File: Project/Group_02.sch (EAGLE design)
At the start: 29 parts, among them J1 POWER_JACKPTH_LOCK, U1 +12v

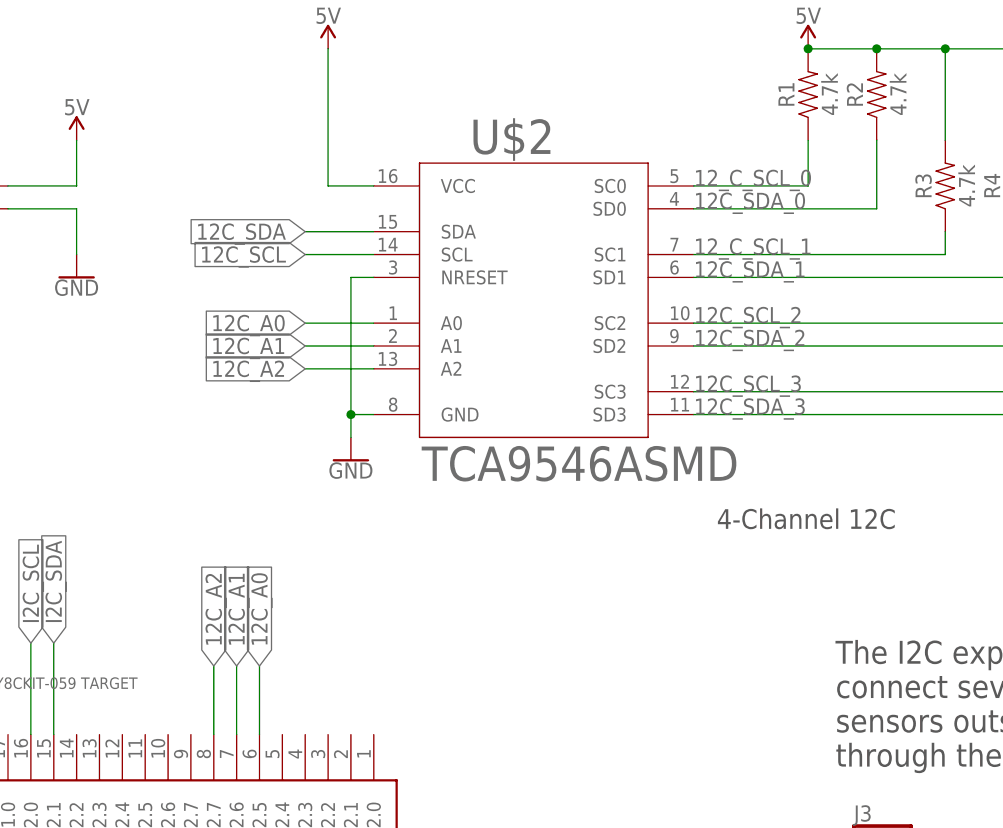
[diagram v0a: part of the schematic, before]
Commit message: PCB completa
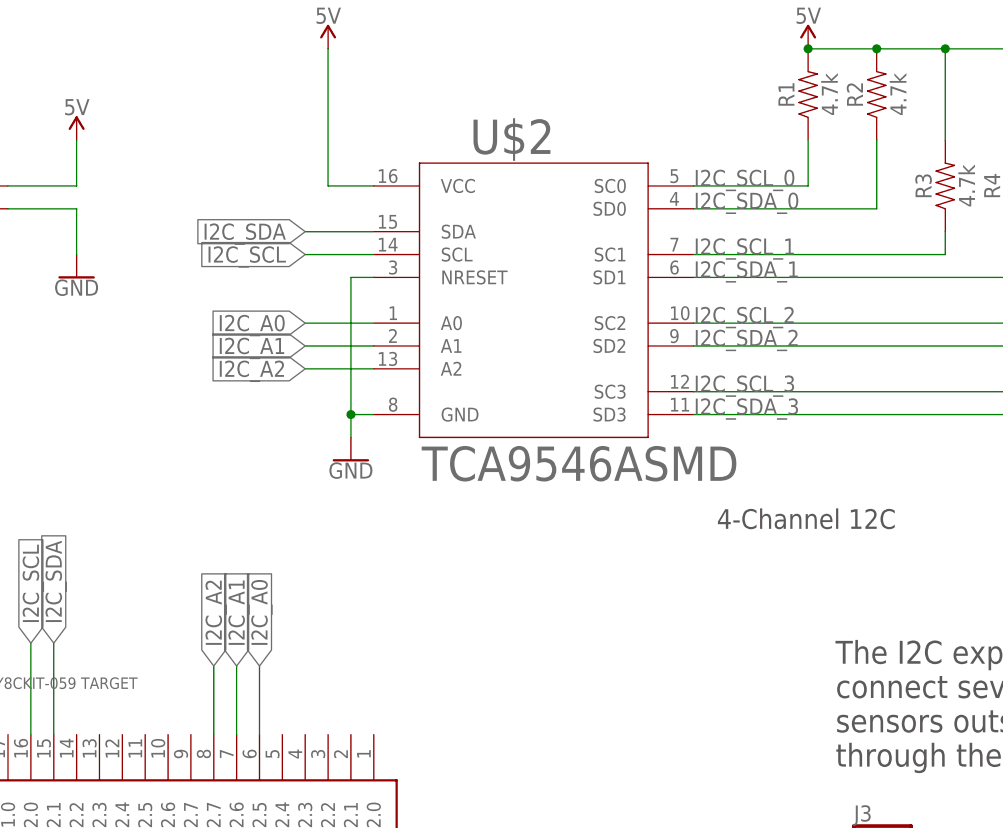
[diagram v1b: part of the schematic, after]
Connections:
- net 12C_A0 renamed I2C_A0
- net 12C_A1 renamed I2C_A1
- net 12C_A2 renamed I2C_A2
- removed net 12C_SCL: U$2.SCL
- removed net 12C_SCL_2: R5.1, U$2.SC2
- removed net 12C_SCL_3: R7.1, U$2.SC3
- removed net 12C_SDA: U$2.SDA
- removed net 12C_SDA_0: R2.1, U$2.SD0
- removed net 12C_SDA_1: R4.1, U$2.SD1
- removed net 12C_SDA_2: R6.1, U$2.SD2
- removed net 12C_SDA_3: R8.1, U$2.SD3
- removed net 12_C_SCL_0: R1.1, U$2.SC0
- removed net 12_C_SCL_1: R3.1, U$2.SC1
- net I2C_SCL: now also U$2.SCL
- net I2C_SCL_0: now also R1.1, U$2.SC0
- net I2C_SCL_1: now also R3.1, U$2.SC1
- net I2C_SCL_2: now also R5.1, U$2.SC2
- net I2C_SCL_3: now also R7.1, U$2.SC3
- net I2C_SDA: now also U$2.SDA
- net I2C_SDA_0: now also R2.1, U$2.SD0
- net I2C_SDA_1: now also R4.1, U$2.SD1
- net I2C_SDA_2: now also R6.1, U$2.SD2
- net I2C_SDA_3: now also R8.1, U$2.SD3
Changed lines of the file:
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@@
 <label x="243.84" y="40.64" size="1.778" layer="95" xref="yes"/>
+</segment>
+<segment>
+<pinref part="U$2" gate="G$1" pin="SD3"/>
+<pinref part="R8" gate="G$1" pin="1"/>
+<wire x1="205.74" y1="137.16" x2="271.78" y2="137.16" width="0.1524" layer="91"/>
+<wire x1="271.78" y1="137.16" x2="271.78" y2="142.24" width="0.1524" layer="91"/>
+<label x="205.74" y="137.16" size="1.778" layer="95"/>
 </segment>
 </net>
@@
 <label x="243.84" y="43.18" size="1.778" layer="95" xref="yes"/>
 </segment>
+<segment>
+<pinref part="U$2" gate="G$1" pin="SC3"/>
+<pinref part="R7" gate="G$1" pin="1"/>
+<wire x1="205.74" y1="139.7" x2="264.16" y2="139.7" width="0.1524" layer="91"/>
+<wire x1="264.16" y1="139.7" x2="264.16" y2="142.24" width="0.1524" layer="91"/>
+<label x="205.74" y="139.7" size="1.778" layer="95"/>
+</segment>
 </net>
 <net name="I2C_SDA_2" class="0">
@@
 <label x="243.84" y="55.88" size="1.778" layer="95" xref="yes"/>
 </segment>
+<segment>
+<pinref part="U$2" gate="G$1" pin="SD2"/>
+<pinref part="R6" gate="G$1" pin="1"/>
+<wire x1="205.74" y1="144.78" x2="256.54" y2="144.78" width="0.1524" layer="91"/>
+<wire x1="256.54" y1="144.78" x2="256.54" y2="149.86" width="0.1524" layer="91"/>
+<label x="205.74" y="144.78" size="1.778" layer="95"/>
+</segment>
 </net>
 <net name="I2C_SCL_2" class="0">
@@
 <label x="243.84" y="58.42" size="1.778" layer="95" xref="yes"/>
 </segment>
+<segment>
+<pinref part="U$2" gate="G$1" pin="SC2"/>
+<pinref part="R5" gate="G$1" pin="1"/>
+<wire x1="205.74" y1="147.32" x2="248.92" y2="147.32" width="0.1524" layer="91"/>
+<wire x1="248.92" y1="147.32" x2="248.92" y2="149.86" width="0.1524" layer="91"/>
+<label x="205.74" y="147.32" size="1.778" layer="95"/>
+</segment>
 </net>
 <net name="I2C_SDA_1" class="0">
@@
 <label x="243.84" y="71.12" size="1.778" layer="95" xref="yes"/>
 </segment>
+<segment>
+<pinref part="U$2" gate="G$1" pin="SD1"/>
+<pinref part="R4" gate="G$1" pin="1"/>
+<wire x1="205.74" y1="152.4" x2="241.3" y2="152.4" width="0.1524" layer="91"/>
+<wire x1="241.3" y1="152.4" x2="241.3" y2="157.48" width="0.1524" layer="91"/>
+<label x="205.74" y="152.4" size="1.778" layer="95"/>
+</segment>
 </net>
 <net name="I2C_SCL_1" class="0">
@@
 <label x="243.84" y="73.66" size="1.778" layer="95" xref="yes"/>
 </segment>
+<segment>
+<pinref part="U$2" gate="G$1" pin="SC1"/>
+<pinref part="R3" gate="G$1" pin="1"/>
+<wire x1="205.74" y1="154.94" x2="233.68" y2="154.94" width="0.1524" layer="91"/>
+<wire x1="233.68" y1="154.94" x2="233.68" y2="157.48" width="0.1524" layer="91"/>
+<label x="205.74" y="154.94" size="1.778" layer="95"/>
+</segment>
 </net>
 <net name="I2C_SDA_0" class="0">
@@
 <label x="243.84" y="86.36" size="1.778" layer="95" xref="yes"/>
 </segment>
+<segment>
+<pinref part="U$2" gate="G$1" pin="SD0"/>
+<pinref part="R2" gate="G$1" pin="1"/>
+<wire x1="205.74" y1="160.02" x2="226.06" y2="160.02" width="0.1524" layer="91"/>
+<wire x1="226.06" y1="160.02" x2="226.06" y2="167.64" width="0.1524" layer="91"/>
+<label x="205.74" y="160.02" size="1.778" layer="95"/>
+</segment>
 </net>
 <net name="I2C_SCL_0" class="0">
@@
 <label x="243.84" y="88.9" size="1.778" layer="95" xref="yes"/>
 </segment>
+<segment>
+<pinref part="U$2" gate="G$1" pin="SC0"/>
+<pinref part="R1" gate="G$1" pin="1"/>
+<wire x1="205.74" y1="162.56" x2="218.44" y2="162.56" width="0.1524" layer="91"/>
+<wire x1="218.44" y1="162.56" x2="218.44" y2="167.64" width="0.1524" layer="91"/>
+<label x="205.74" y="162.56" size="1.778" layer="95"/>
+</segment>
 </net>
 <net name="MUX_A0/2.3C" class="0">
@@
 <label x="132.08" y="111.76" size="1.778" layer="95" rot="R90" xref="yes"/>
 </segment>
+<segment>
+<pinref part="U$2" gate="G$1" pin="SCL"/>
+<wire x1="170.18" y1="154.94" x2="162.56" y2="154.94" width="0.1524" layer="91"/>
+<label x="162.56" y="154.94" size="1.778" layer="95" rot="R180" xref="yes"/>
+</segment>
 </net>
 <net name="I2C_SDA" class="0">
@@
 <wire x1="134.62" y1="101.6" x2="134.62" y2="111.76" width="0.1524" layer="91"/>
 <label x="134.62" y="111.76" size="1.778" layer="95" rot="R90" xref="yes"/>
+</segment>
+<segment>
+<pinref part="U$2" gate="G$1" pin="SDA"/>
+<wire x1="170.18" y1="157.48" x2="162.56" y2="157.48" width="0.1524" layer="91"/>
+<label x="162.56" y="157.48" size="1.778" layer="95" rot="R180" xref="yes"/>
 </segment>
 </net>
@@
 </segment>
 </net>
-<net name="12_C_SCL_0" class="0">
-<segment>
-<pinref part="U$2" gate="G$1" pin="SC0"/>
-<pinref part="R1" gate="G$1" pin="1"/>
-<wire x1="205.74" y1="162.56" x2="218.44" y2="162.56" width="0.1524" layer="91"/>
-<wire x1="218.44" y1="162.56" x2="218.44" y2="167.64" width="0.1524" layer="91"/>
-<label x="205.74" y="162.56" size="1.778" layer="95"/>
-</segment>
-</net>
-<net name="12C_SDA_0" class="0">
-<segment>
-<pinref part="U$2" gate="G$1" pin="SD0"/>
-<pinref part="R2" gate="G$1" pin="1"/>
-<wire x1="205.74" y1="160.02" x2="226.06" y2="160.02" width="0.1524" layer="91"/>
-<wire x1="226.06" y1="160.02" x2="226.06" y2="167.64" width="0.1524" layer="91"/>
-<label x="205.74" y="160.02" size="1.778" layer="95"/>
-</segment>
-</net>
-<net name="12_C_SCL_1" class="0">
-<segment>
-<pinref part="U$2" gate="G$1" pin="SC1"/>
-<pinref part="R3" gate="G$1" pin="1"/>
-<wire x1="205.74" y1="154.94" x2="233.68" y2="154.94" width="0.1524" layer="91"/>
-<wire x1="233.68" y1="154.94" x2="233.68" y2="157.48" width="0.1524" layer="91"/>
-<label x="205.74" y="154.94" size="1.778" layer="95"/>
-</segment>
-</net>
-<net name="12C_SDA_1" class="0">
-<segment>
-<pinref part="U$2" gate="G$1" pin="SD1"/>
-<pinref part="R4" gate="G$1" pin="1"/>
-<wire x1="205.74" y1="152.4" x2="241.3" y2="152.4" width="0.1524" layer="91"/>
-<wire x1="241.3" y1="152.4" x2="241.3" y2="157.48" width="0.1524" layer="91"/>
-<label x="205.74" y="152.4" size="1.778" layer="95"/>
-</segment>
-</net>
-<net name="12C_SCL_2" class="0">
-<segment>
-<pinref part="U$2" gate="G$1" pin="SC2"/>
-<pinref part="R5" gate="G$1" pin="1"/>
-<wire x1="205.74" y1="147.32" x2="248.92" y2="147.32" width="0.1524" layer="91"/>
-<wire x1="248.92" y1="147.32" x2="248.92" y2="149.86" width="0.1524" layer="91"/>
-<label x="205.74" y="147.32" size="1.778" layer="95"/>
-</segment>
-</net>
-<net name="12C_SDA_2" class="0">
-<segment>
-<pinref part="U$2" gate="G$1" pin="SD2"/>
-<pinref part="R6" gate="G$1" pin="1"/>
-<wire x1="205.74" y1="144.78" x2="256.54" y2="144.78" width="0.1524" layer="91"/>
-<wire x1="256.54" y1="144.78" x2="256.54" y2="149.86" width="0.1524" layer="91"/>
-<label x="205.74" y="144.78" size="1.778" layer="95"/>
-</segment>
-</net>
-<net name="12C_SCL_3" class="0">
-<segment>
-<pinref part="U$2" gate="G$1" pin="SC3"/>
-<pinref part="R7" gate="G$1" pin="1"/>
-<wire x1="205.74" y1="139.7" x2="264.16" y2="139.7" width="0.1524" layer="91"/>
-<wire x1="264.16" y1="139.7" x2="264.16" y2="142.24" width="0.1524" layer="91"/>
-<label x="205.74" y="139.7" size="1.778" layer="95"/>
-</segment>
-</net>
-<net name="12C_SDA_3" class="0">
-<segment>
-<pinref part="U$2" gate="G$1" pin="SD3"/>
-<pinref part="R8" gate="G$1" pin="1"/>
-<wire x1="205.74" y1="137.16" x2="271.78" y2="137.16" width="0.1524" layer="91"/>
-<wire x1="271.78" y1="137.16" x2="271.78" y2="142.24" width="0.1524" layer="91"/>
-<label x="205.74" y="137.16" size="1.778" layer="95"/>
-</segment>
-</net>
-<net name="12C_SDA" class="0">
-<segment>
-<pinref part="U$2" gate="G$1" pin="SDA"/>
-<wire x1="170.18" y1="157.48" x2="162.56" y2="157.48" width="0.1524" layer="91"/>
-<label x="162.56" y="157.48" size="1.778" layer="95" rot="R180" xref="yes"/>
-</segment>
-</net>
-<net name="12C_SCL" class="0">
-<segment>
-<pinref part="U$2" gate="G$1" pin="SCL"/>
-<wire x1="170.18" y1="154.94" x2="162.56" y2="154.94" width="0.1524" layer="91"/>
-<label x="162.56" y="154.94" size="1.778" layer="95" rot="R180" xref="yes"/>
-</segment>
-</net>
-<net name="12C_A0" class="0">
+<net name="I2C_A0" class="0">
 <segment>
 <pinref part="U$2" gate="G$1" pin="A0"/>
@@
 </segment>
 </net>
-<net name="12C_A1" class="0">
+<net name="I2C_A1" class="0">
 <segment>
 <pinref part="U$2" gate="G$1" pin="A1"/>
@@
 </segment>
 </net>
-<net name="12C_A2" class="0">
+<net name="I2C_A2" class="0">
 <segment>
 <pinref part="U$2" gate="G$1" pin="A2"/>

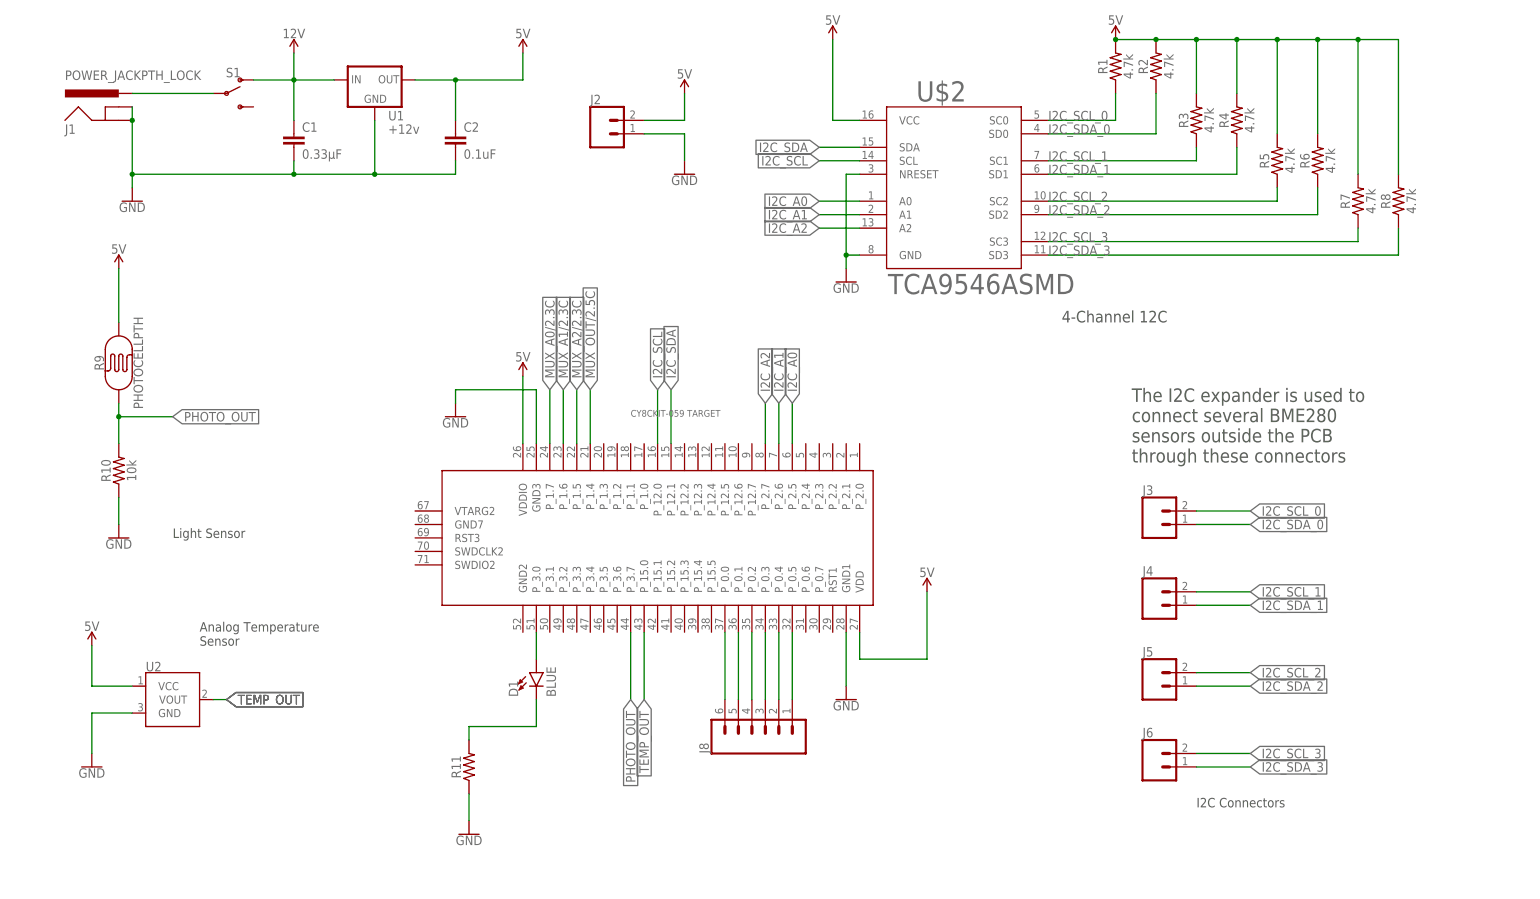
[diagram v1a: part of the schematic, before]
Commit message: Aggiornamento schematico
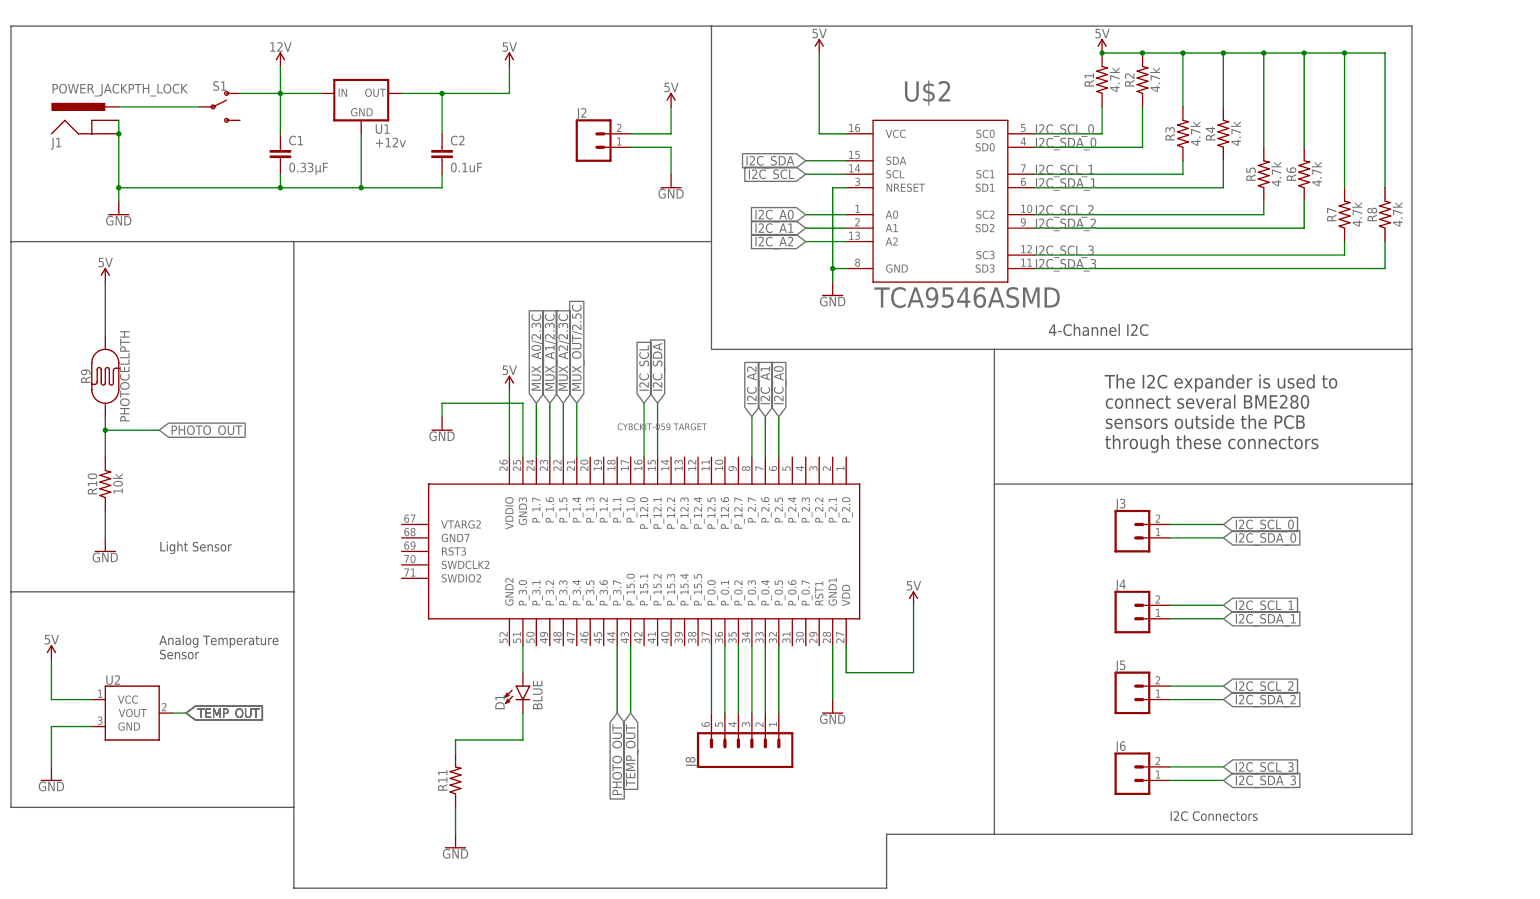
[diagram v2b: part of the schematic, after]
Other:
- note added: "4-Channel I2C"
- note removed: "4-Channel 12C"
- moved on the sheet: C1, C2, D1, J1, J2, J3, J4, J5, J6, J8, R1, R10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
